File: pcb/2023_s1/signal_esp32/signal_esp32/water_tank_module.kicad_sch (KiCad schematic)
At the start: 14 parts, among them J1 Screw_Terminal_01x02, J3 Screw_Terminal_01x05, U4 NRF24L01_Breakout

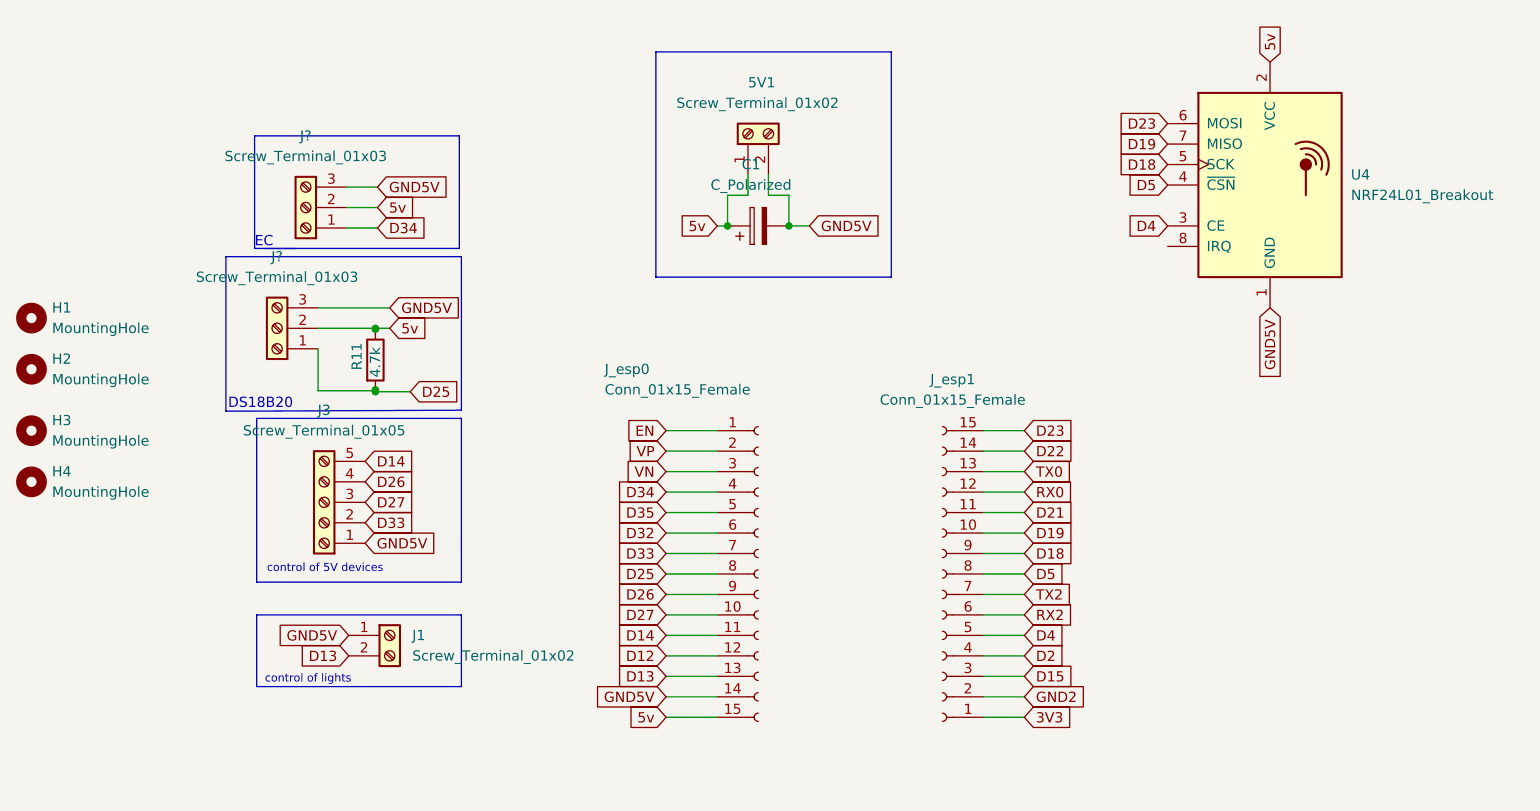
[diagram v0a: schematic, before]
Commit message: update
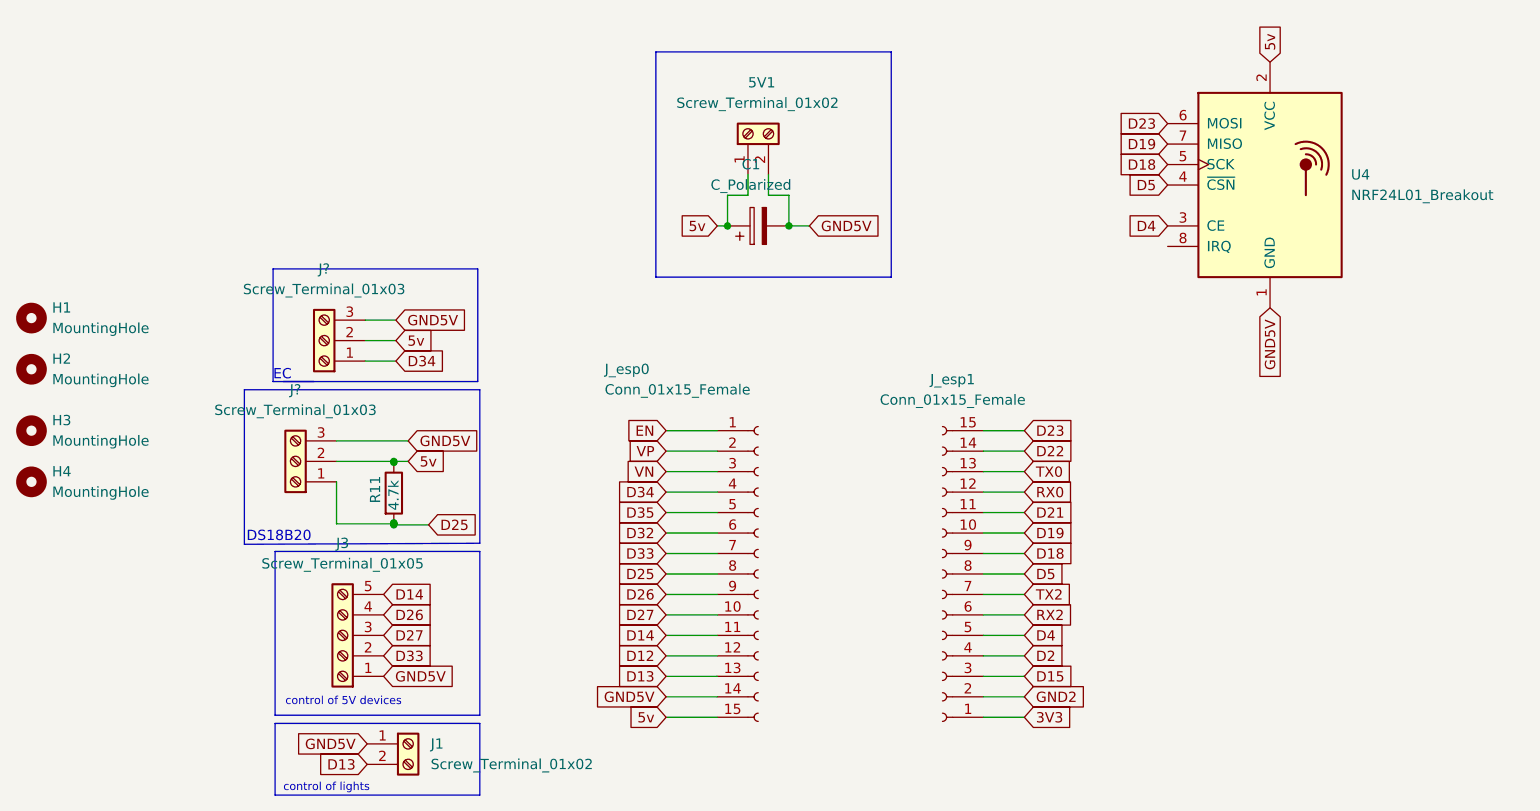
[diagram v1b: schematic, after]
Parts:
- J1: footprint (none) -> TerminalBlock_Altech:Altech_AK300_1x02_P5.00mm_45-Degree
- J?: footprint (none) -> TerminalBlock_Altech:Altech_AK300_1x03_P5.00mm_45-Degree
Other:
- moved on the sheet: J1, J3, J?, R11
